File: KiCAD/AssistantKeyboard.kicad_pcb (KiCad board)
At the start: 2 copper layers, 64 x 108 mm, 14 parts, among them J1 Conn_01x04_Male, J2 Conn_01x12_Male, J3 Conn_01x12_Male, J4 Conn_01x02_Male, SW1 SW_Push, SW13 RotaryEncoder_Switch, SW2 SW_Push, SW3 SW_Push, SW4 SW_Push, SW5 SW_Push, SW6 SW_Push, SW7 SW_Push, SW8 SW_Push, SW9 SW_Push

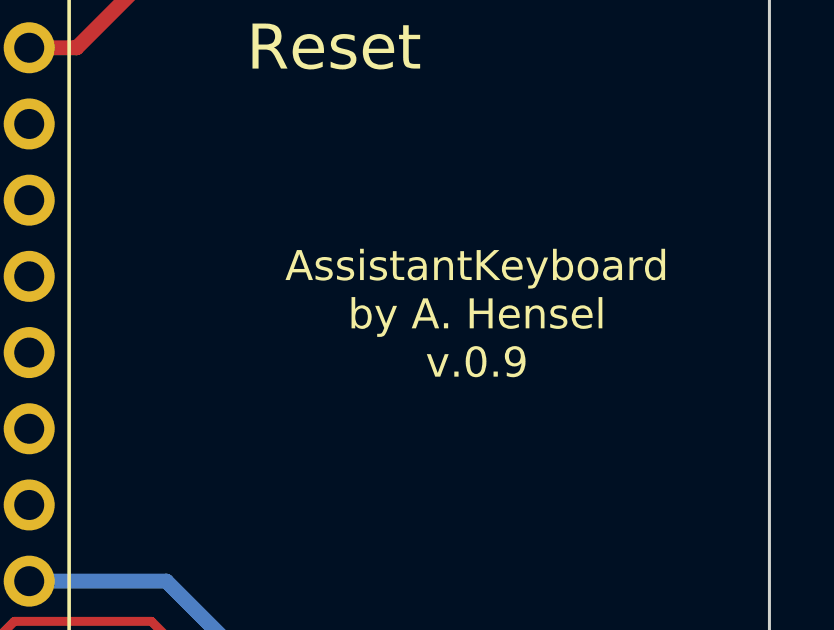
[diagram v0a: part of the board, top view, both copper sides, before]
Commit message: V1.0
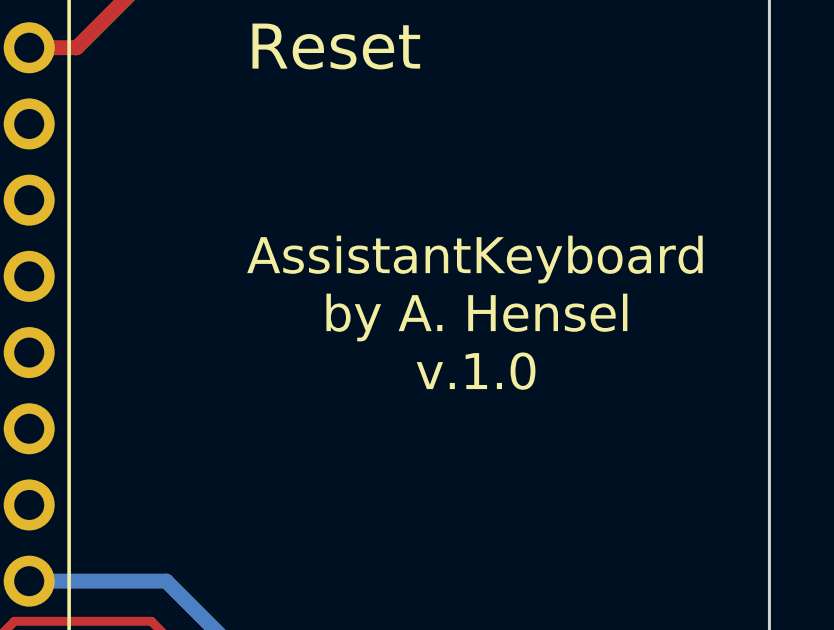
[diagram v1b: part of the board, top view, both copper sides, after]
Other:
- board text added: "AssistantKeyboard by A. Hensel v.1.0"
- board text removed: "AssistantKeyboard by A. Hensel v.0.9"
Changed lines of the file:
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@@
     (effects (font (size 1.5 1.5) (thickness 0.3)))
   )
-  (gr_text "AssistantKeyboard\nby A. Hensel\nv.0.9" (at 111.252 49.53) (layer "F.SilkS")
-    (effects (font (size 1 1) (thickness 0.15)))
+  (gr_text "AssistantKeyboard\nby A. Hensel\nv.1.0" (at 111.252 49.53) (layer "F.SilkS")
+    (effects (font (size 1.2 1.2) (thickness 0.15)))
   )
   (gr_text "Display I²C" (at 115.57 66.802 90) (layer "F.SilkS")
